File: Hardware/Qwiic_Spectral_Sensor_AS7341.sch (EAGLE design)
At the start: 21 parts, among them J1 QWIIC_RIGHT_ANGLE, J3 QWIIC_RIGHT_ANGLE, U1 MLX90614

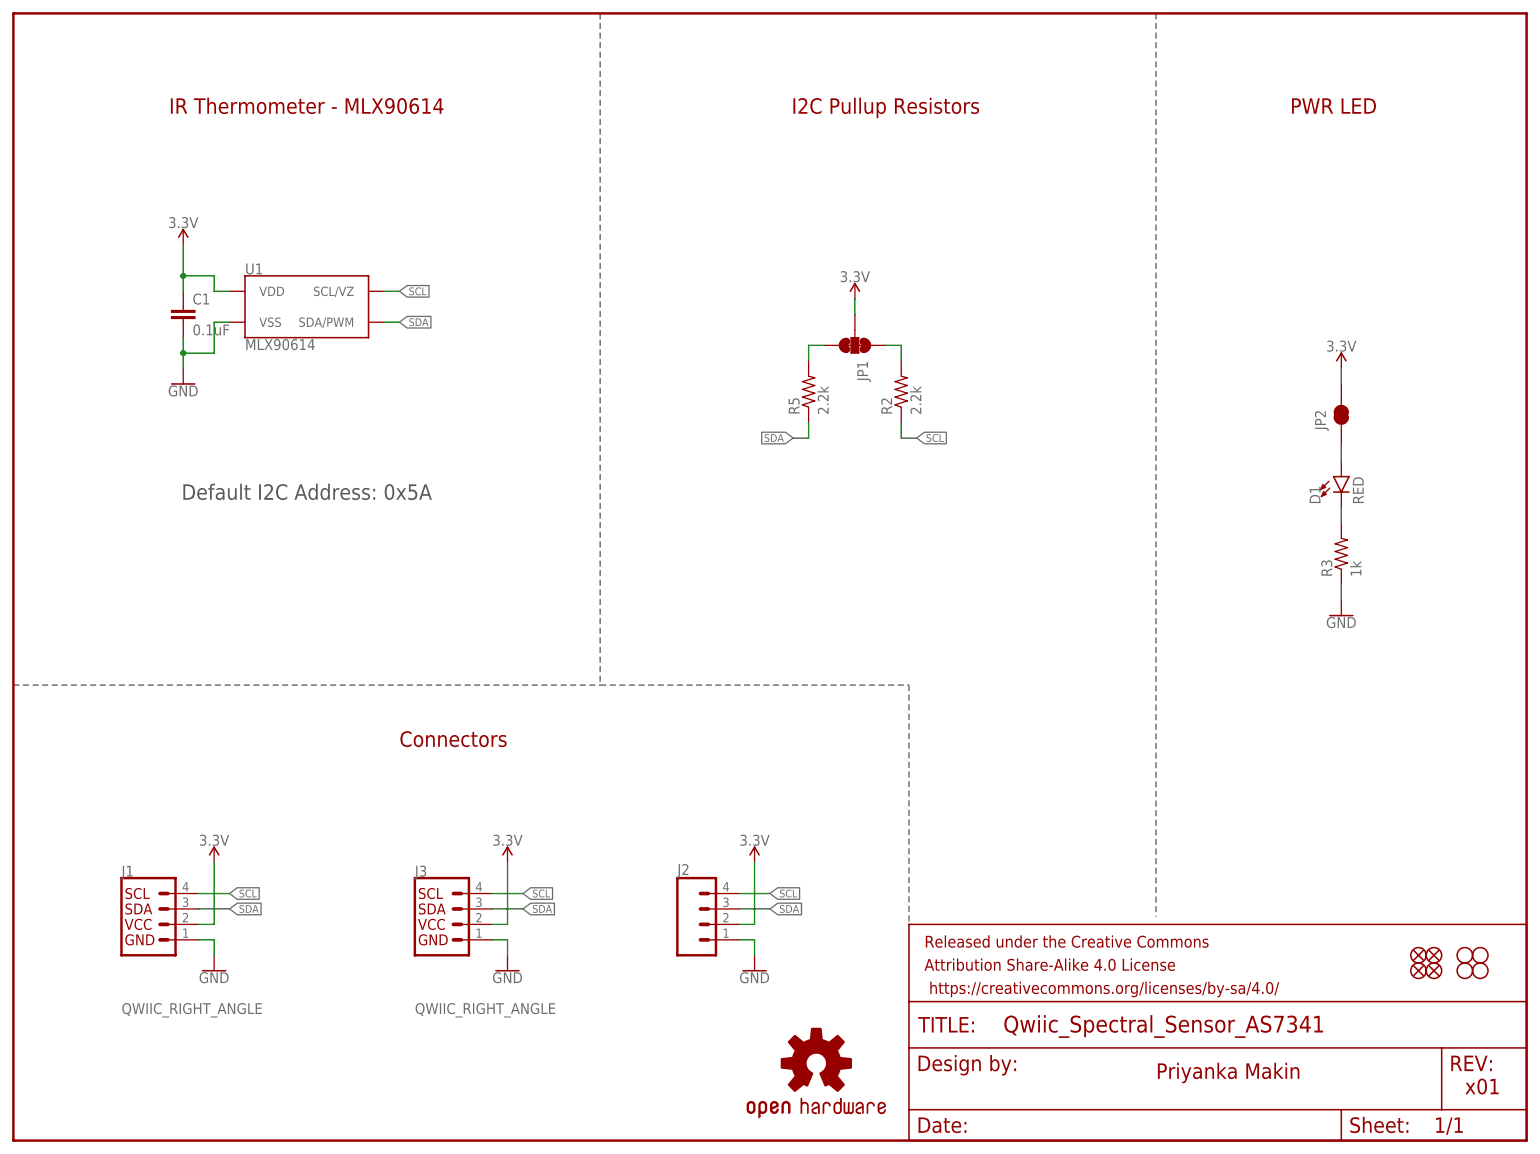
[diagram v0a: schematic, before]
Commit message: Working on schematic
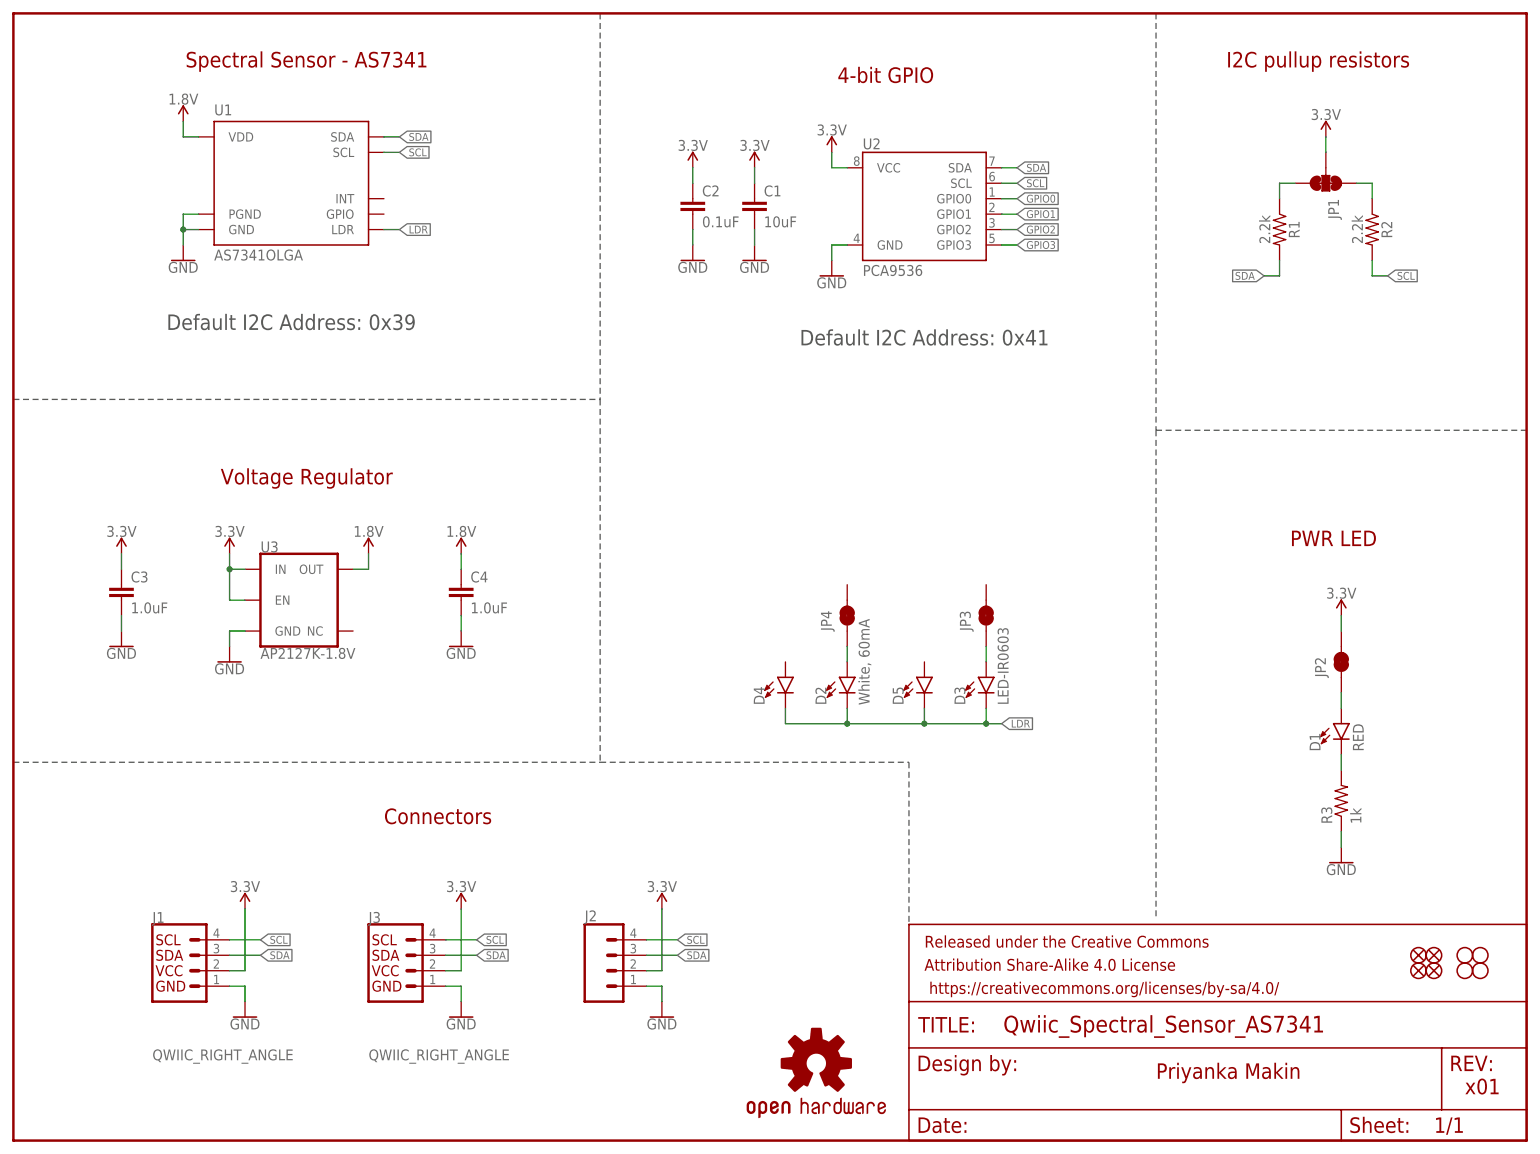
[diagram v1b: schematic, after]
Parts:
- removed R5: 2.2k, SparkFun-Resistors:2.2KOHM-0603-1/10W-1%
- added C2: 0.1uF, SparkFun-Capacitors:0.1UF-0603-25V-(+80/-20%)
- added C3, C4: 1.0uF, SparkFun-Capacitors:1.0UF-0603-16V-10%
- added D2: White, 60mA, SparkFun-LED:LED-WHITE3014
- added D3: LED-IR0603, SparkFun-LED:LED-IR0603
- added D4, D5: (no value), SparkFun-LED:LED-3MM-NO_SILK
- added JP3, JP4: JUMPER-SMT_2_NC_TRACE_SILK, SparkFun-Jumpers:JUMPER-SMT_2_NC_TRACE_SILK
- added R1: 2.2k, SparkFun-Resistors:2.2KOHM-0603-1/10W-1%
- added U2: PCA9536, New_Parts:PCA9536
- added U3: AP2127K-1.8V, SparkFun-IC-Power:V_REG_AP2127K-1.8V
- C1: value 0.1uF -> 10uF; device SparkFun-Capacitors:0.1UF-0603-25V-5% -> SparkFun-Capacitors:10UF-0603-6.3V-20%
- U1: value MLX90614 -> AS7341OLGA; device SparkFun-Sensors:MLX90614 -> AS7341:AS7341OLGA
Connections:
- new net 1.8V: C4.1, U1.VDD, U3.OUT
- new net GPIO0: U2.GPIO0
- new net GPIO1: U2.GPIO1
- new net GPIO2: U2.GPIO2
- new net GPIO3: U2.GPIO3
- new net LDR: D2.C, D3.C, D4.C, D5.C, U1.LDR
- new net N$5: D2.A, JP4.1
- new net N$6: U3.EN, U3.IN
- new net N$7: D3.A, JP3.1
- net 3.3V: now also C2.1, C3.1, U2.VCC; no longer U1.VDD
- net GND: now also C2.2, C3.2, C4.2, U1.GND, U1.PGND, U2.GND, U3.GND; no longer U1.VSS
- net N$1: now also JP1.3, R1.1; no longer JP1.1, R2.2
- net N$3: now also JP1.1, R2.1; no longer JP1.3, R5.2
- net SCL: now also R2.2, U1.SCL, U2.SCL; no longer R2.1, U1.SCL/VZ
- net SDA: now also R1.2, U1.SDA, U2.SDA; no longer R5.1, U1.SDA/PWM
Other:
- note added: "4-bit GPIO"
- note added: "Default I2C Address: 0x39"
- note added: "Default I2C Address: 0x41"
- note added: "I2C pullup resistors"
- note added: "Spectral Sensor - AS7341"
- note added: "Voltage Regulator"
- note removed: "Default I2C Address: 0x5A"
- note removed: "I2C Pullup Resistors"
- note removed: "IR Thermometer - MLX90614"
- moved on the sheet: C1, D1, J1, J2, J3, JP1, JP2, R2, R3
